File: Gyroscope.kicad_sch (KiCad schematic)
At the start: 29 parts, among them J1 Barrel_Jack_Switch, J2 Micro_SD_Card_Det2, U1 IIS3DWB, U2 APS6404L-3SQRx-SN, U3 STM32G431C6Tx, U4 W25Q128JVS, U5 CR2013-MI2120, U6 AP2112K-3.3, U7 74LVC1G139

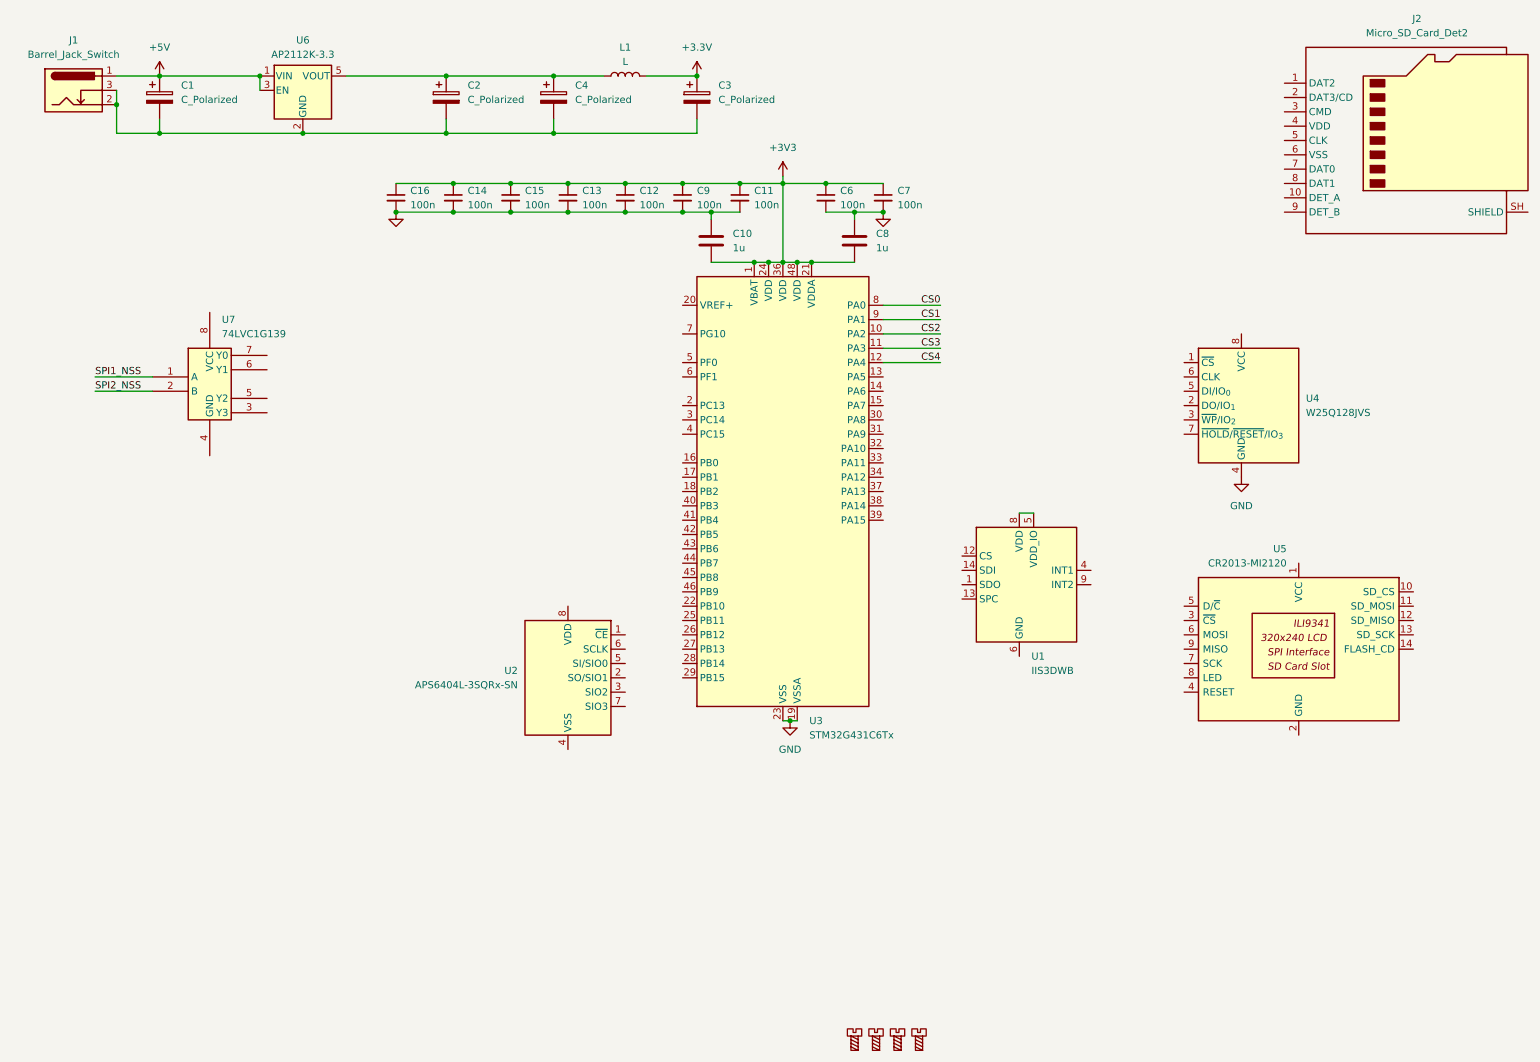
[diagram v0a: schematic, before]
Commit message: refresh
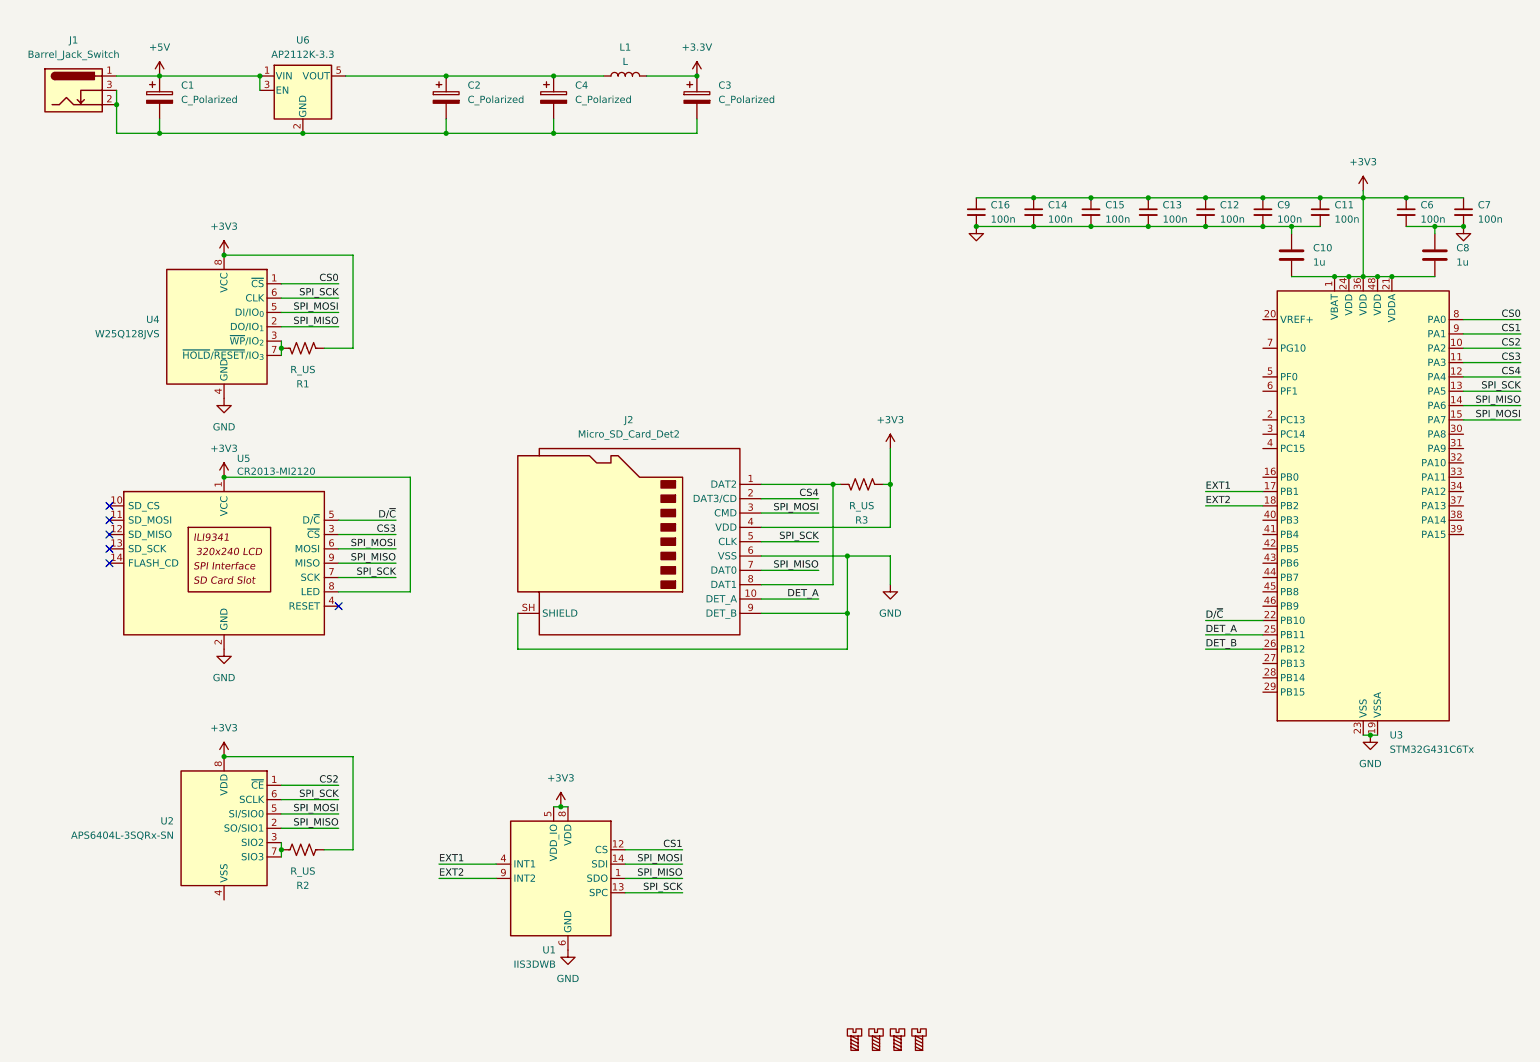
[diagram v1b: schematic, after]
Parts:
- removed U7: 74LVC1G139, Package_SO:VSSOP-8_2.3x2mm_P0.5mm, symbol 74xGxx:74LVC1G139
- added R1, R2, R3: R_US, symbol Device:R_US
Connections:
- net +3V3: now also J2.4 (VDD), U1.5 (VDD_IO), U1.8 (VDD), U2.8 (VDD), U4.8 (VCC), U5.1 (VCC), U5.8 (LED), R1.1, R2.2, R3.1
- net CS0: now also U4.1 (~{CS})
- net CS1: now also U1.12 (CS)
- net CS2: now also U2.1 (~{CE})
- net CS3: now also U5.3 (~{CS})
- net CS4: now also J2.2 (DAT3/CD)
- net GND: now also J2.6 (VSS), J2.9 (DET_B), J2.SH (SHIELD), U1.2 (GND), U1.3 (GND), U1.6 (GND), U1.7 (GND), U5.2 (GND)
- net D/~{C}: now reaches U5.5 (D/~{C})
- net D/~{C}: now also U3.22 (PB10)
- net SPI_MOSI: now reaches U5.6 (MOSI)
- net SPI_MOSI: now also J2.3 (CMD), U1.14 (SDI), U2.5 (SI/SIO0), U3.15 (PA7), U4.5 (DI/IO_{0})
- net SPI_SCK: now reaches U5.7 (SCK)
- net SPI_SCK: now also J2.5 (CLK), U1.13 (SPC), U2.6 (SCLK), U3.13 (PA5), U4.6 (CLK)
- net SPI_MISO: now reaches U5.9 (MISO)
- net SPI_MISO: now also J2.7 (DAT0), U1.1 (SDO), U2.2 (SO/SIO1), U3.14 (PA6), U4.2 (DO/IO_{1})
- net at U2.3 (SIO2): now also U2.7 (SIO3), R2.1
- net EXT1: now reaches U3.17 (PB1)
- net EXT1: now also U1.4 (INT1)
- net EXT2: now reaches U3.18 (PB2)
- net EXT2: now also U1.9 (INT2)
- net DET_A: now reaches U3.25 (PB11)
- net DET_A: now also J2.10 (DET_A)
- net DET_B: now reaches U3.26 (PB12)
- net at U4.3 (~{WP}/IO_{2}): now also U4.7 (~{HOLD}/~{RESET}/IO_{3}), R1.2
- net at J2.1 (DAT2): now also J2.8 (DAT1), R3.2
- no-connect marks 0 -> 6
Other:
- moved on the sheet: C10, C11, C12, C13, C14, C15, C16, C6, C7, C8, C9, J2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

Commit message: refresh
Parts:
- C1, C2, C3, C4: footprint (none) -> Capacitor_Tantalum_SMD:CP_EIA-3528-12_Kemet-T
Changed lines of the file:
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@@
 			)
 		)
-		(property "Footprint" ""
+		(property "Footprint" "Capacitor_Tantalum_SMD:CP_EIA-3528-12_Kemet-T"
 			(at 40.3352 30.48 0)
 			(hide yes)
@@
 			)
 		)
-		(property "Footprint" ""
+		(property "Footprint" "Capacitor_Tantalum_SMD:CP_EIA-3528-12_Kemet-T"
 			(at 110.1852 30.48 0)
 			(hide yes)
@@
 			)
 		)
-		(property "Footprint" ""
+		(property "Footprint" "Capacitor_Tantalum_SMD:CP_EIA-3528-12_Kemet-T"
 			(at 91.1352 30.48 0)
 			(hide yes)
@@
 			)
 		)
-		(property "Footprint" ""
+		(property "Footprint" "Capacitor_Tantalum_SMD:CP_EIA-3528-12_Kemet-T"
 			(at 135.5852 30.48 0)
 			(hide yes)
